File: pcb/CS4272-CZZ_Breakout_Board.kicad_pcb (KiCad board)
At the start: 2 copper layers, 141.1 x 78.5 mm, 162 parts, among them J1 Conn_01x14, J2 Conn_01x12, Q1 AO3401A, U1 CS4272, U2 SPX3819M5-L-3-3, U3 NE5532, U4 NE5532, U5 NE5532, U6 NE5532, U7 NE5532, U8 NE5532, Y1 24.576 MHz

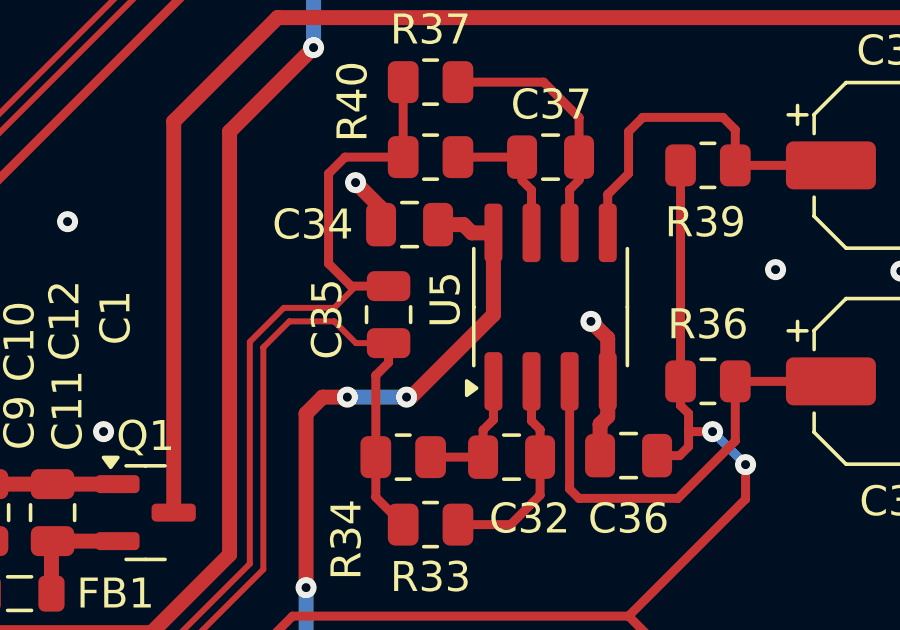
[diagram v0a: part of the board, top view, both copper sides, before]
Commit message: PCB update
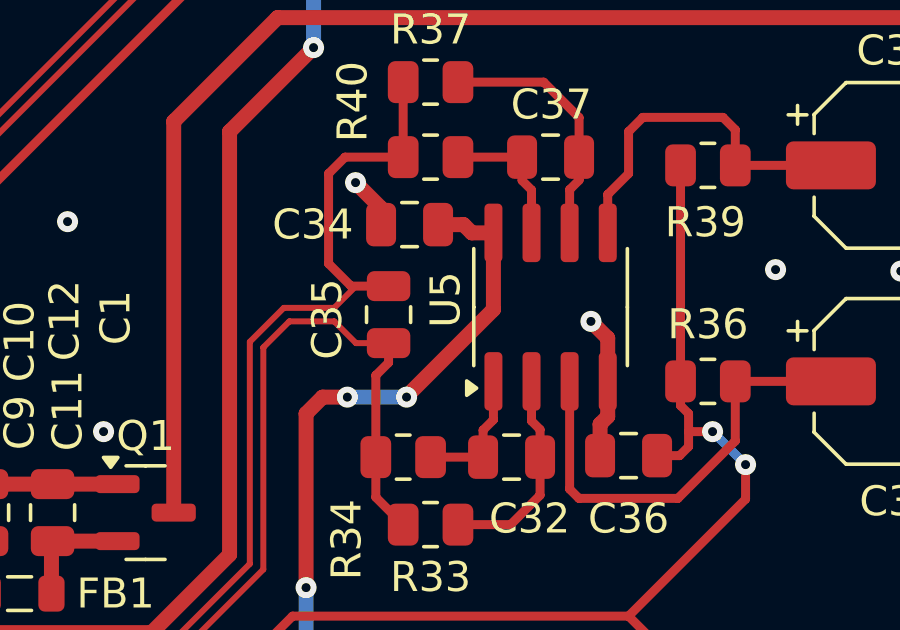
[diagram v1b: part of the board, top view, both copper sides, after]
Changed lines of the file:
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@@
 			(psa4output no)
 			(plotreference yes)
-			(plotvalue yes)
+			(plotvalue no)
 			(plotfptext yes)
 			(plotinvisibletext no)
 			(sketchpadsonfab no)
-			(subtractmaskfromsilk no)
+			(subtractmaskfromsilk yes)
 			(outputformat 1)
 			(mirror no)
-			(drillshape 1)
+			(drillshape 0)
 			(scaleselection 1)
-			(outputdirectory "")
+			(outputdirectory "Manufacturing/")
 		)
 	)
@@
 	)
 	(segment
-		(start 147.22 103.755)
+		(start 147.22 103.58)
 		(end 147.22 101.025)
 		(width 0.5)
@@
 	)
 	(segment
+		(start 144.325 106.475)
+		(end 147.22 103.58)
+		(width 0.5)
+		(layer "F.Cu")
+		(net 1)
+	)
+	(segment
 		(start 178.07 122.005)
 		(end 178.07 122.6575)
@@
 	)
 	(segment
-		(start 144.475 106.5)
-		(end 147.22 103.755)
-		(width 0.5)
-		(layer "F.Cu")
-		(net 1)
-	)
-	(segment
 		(start 140.975 107.05)
 		(end 140.975 112.85)
@@
 	)
 	(segment
-		(start 144.325 106.5)
-		(end 144.475 106.5)
-		(width 0.5)
-		(layer "F.Cu")
-		(net 1)
-	)
-	(segment
 		(start 139.925 121.65)
 		(end 139.325 121.65)
@@
 	)
 	(segment
+		(start 144.325 106.5)
+		(end 144.325 106.475)
+		(width 0.5)
+		(layer "F.Cu")
+		(net 1)
+	)
+	(segment
 		(start 141.225 71.65)
 		(end 147.875 71.65)
@@
 	)
 	(zone
+		(net 0)
+		(net_name "")
+		(layer "F.Cu")
+		(hatch edge 0.5)
+		(connect_pads
+			(clearance 0)
+		)
+		(min_thickness 0.25)
+		(filled_areas_thickness no)
+		(keepout
+			(tracks allowed)
+			(vias allowed)
+			(pads allowed)
+			(copperpour not_allowed)
+			(footprints allowed)
+		)
+		(fill
+			(thermal_gap 0.5)
+			(thermal_bridge_width 0.5)
+		)
+		(polygon
+			(pts
+				(xy 132.3 126.9) (xy 129.3 123.9) (xy 129.8 123.5) (xy 132.8 126.5)
+			)
+		)
+	)
+	(zone
+		(net 0)
+		(net_name "")
+		(layer "F.Cu")
+		(hatch edge 0.5)
+		(connect_pads
+			(clearance 0)
+		)
+		(min_thickness 0.25)
+		(filled_areas_thickness no)
+		(keepout
+			(tracks allowed)
+			(vias allowed)
+			(pads allowed)
+			(copperpour not_allowed)
+			(footprints allowed)
+		)
+		(fill
+			(thermal_gap 0.5)
+			(thermal_bridge_width 0.5)
+		)
+		(polygon
+			(pts
+				(xy 130.3 122.6) (xy 131.2 122.3) (xy 136.3 127.5) (xy 135.8 128.2)
+			)
+		)
+	)
+	(zone
+		(net 0)
+		(net_name "")
+		(layer "F.Cu")
+		(hatch edge 0.5)
+		(connect_pads
+			(clearance 0)
+		)
+		(min_thickness 0.25)
+		(filled_areas_thickness no)
+		(keepout
+			(tracks allowed)
+			(vias allowed)
+			(pads allowed)
+			(copperpour not_allowed)
+			(footprints allowed)
+		)
+		(fill
+			(thermal_gap 0.5)
+			(thermal_bridge_width 0.5)
+		)
+		(polygon
+			(pts
+				(xy 195.6 95.6) (xy 195.7 97.7) (xy 202 103.7) (xy 203 102.8)
+			)
+		)
+	)
+	(zone
+		(net 0)
+		(net_name "")
+		(layer "F.Cu")
+		(hatch edge 0.5)
+		(connect_pads
+			(clearance 0)
+		)
+		(min_thickness 0.25)
+		(filled_areas_thickness no)
+		(keepout
+			(tracks allowed)
+			(vias allowed)
+			(pads allowed)
+			(copperpour not_allowed)
+			(footprints allowed)
+		)
+		(fill
+			(thermal_gap 0.5)
+			(thermal_bridge_width 0.5)
+		)
+		(polygon
+			(pts
+				(xy 201.5 99.2) (xy 201.5 96.9) (xy 182.9 78.6) (xy 182.4 79.7) (xy 201.1 99.3)
+			)
+		)
+	)
+	(zone
+		(net 0)
+		(net_name "")
+		(layer "F.Cu")
+		(hatch edge 0.5)
+		(connect_pads
+			(clearance 0)
+		)
+		(min_thickness 0.25)
+		(filled_areas_thickness no)
+		(keepout
+			(tracks allowed)
+			(vias allowed)
+			(pads allowed)
+			(copperpour not_allowed)
+			(footprints allowed)
+		)
+		(fill
+			(thermal_gap 0.5)
+			(thermal_bridge_width 0.5)
+		)
+		(polygon
+			(pts
+				(xy 142.1 98.9) (xy 143.3 98.9) (xy 143.3 100) (xy 142.1 100)
+			)
+		)
+	)
+	(zone
